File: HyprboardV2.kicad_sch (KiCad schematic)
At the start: 0 parts

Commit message: Crystal Oscilator, Flash Memory done! Started working on the breakout for GPIO pins
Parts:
- added C1, C11, C12, C2, C3, C4, C5, C6, C7, C8, C9: 0.1uF, symbol Device:C
- added C10: 1uF, symbol Device:C
- added C13, C14: 10uF, symbol Device:C
- added C15, C16: 15pF, symbol Device:C
- added J1: USB_C_Receptacle_USB2.0_14P, symbol Connector:USB_C_Receptacle_USB2.0_14P
- added R1, R2: 5.1K, symbol Device:R
- added R3, R4: 27, symbol Device:R
- added R5, R7: 1K, symbol Device:R
- added R6: 10K, symbol Device:R
- added SW1: SW_Push, symbol Switch:SW_Push
- added U1: RP2040, Package_DFN_QFN:QFN-56-1EP_7x7mm_P0.4mm_EP3.2x3.2mm, symbol MCU_RaspberryPi:RP2040
- added U2: NCP1117-3.3_SOT223, Package_TO_SOT_SMD:SOT-223-3_TabPin2, symbol Regulator_Linear:NCP1117-3.3_SOT223
- added U3: W25Q128JVS, Package_SO:SOIC-8_5.3x5.3mm_P1.27mm, symbol Memory_Flash:W25Q128JVS
- added Y1: 12 MHz, symbol Device:Crystal_GND24
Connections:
- new net: J1.A5 (CC1), R1.1
- new net: R3.1, U1.46 (USB_DM)
- new net: R4.1, U1.47 (USB_DP)
- new net: R7.1, SW1.2
- new net: C16.2, R5.1, Y1.1
- new net: C13.2, C14.2
- new net: J1.B5 (CC2), R2.1
- new net +1V1: C10.1, C11.1, C12.1, U1.43 (ADC_AVDD), U1.48 (USB_VDD)
- new net +3V3: C1.1, C14.1, C2.1, C3.1, C4.1, C5.1, C6.1, C7.1, C8.1, C9.1, R6.1, U1.1 (IOVDD), U1.10 (IOVDD), U1.22 (IOVDD), U1.23 (DVDD), U1.33 (IOVDD), U1.42 (IOVDD), U1.44 (VREG_VIN), U1.45 (VREG_VOUT), U1.49 (IOVDD), U1.50 (DVDD), U2.2 (VO), U3.8 (VCC)
- new net GND: C1.2, C10.2, C11.2, C12.2, C15.1, C16.1, C2.2, C3.2, C4.2, C5.2, C6.2, C7.2, C8.2, C9.2, J1.A1 (GND), J1.A12 (GND), J1.B1 (GND), J1.B12 (GND), J1.S1 (SHIELD), R1.2, R2.2, SW1.1, U2.1 (GND), U3.4 (GND), Y1.2 (G), Y1.4 (G)
- new net QSPI_SCLK: U1.52 (QSPI_SCLK), U3.6 (CLK)
- new net QSPI_SD0: U1.53 (QSPI_SD0), U3.5 (DI/IO_{0})
- new net QSPI_SD1: U1.55 (QSPI_SD1), U3.2 (DO/IO_{1})
- new net QSPI_SD2: U1.54 (QSPI_SD2), U3.3 (~{WP}/IO_{2})
- new net QSPI_SD3: U1.51 (QSPI_SD3), U3.7 (~{HOLD}/~{RESET}/IO_{3})
- new net QSPI_SS: R6.2, R7.2, U1.56 (~{QSPI_SS}), U3.1 (~{CS})
- new net USD_D+: J1.A6 (D+), J1.B6 (D+), R3.2
- new net USD_D-: J1.A7 (D-), J1.B7 (D-), R4.2
- new net VBUS: C13.1, J1.A4 (VBUS), J1.A9 (VBUS), J1.B4 (VBUS), J1.B9 (VBUS), U2.3 (VI)
- new net XIN: C15.2, U1.20 (XIN), Y1.3
- new net XOUT: R5.2, U1.21 (XOUT)
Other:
- note added: "CRYSTAL OSCILLATOR"
- note added: "USB"

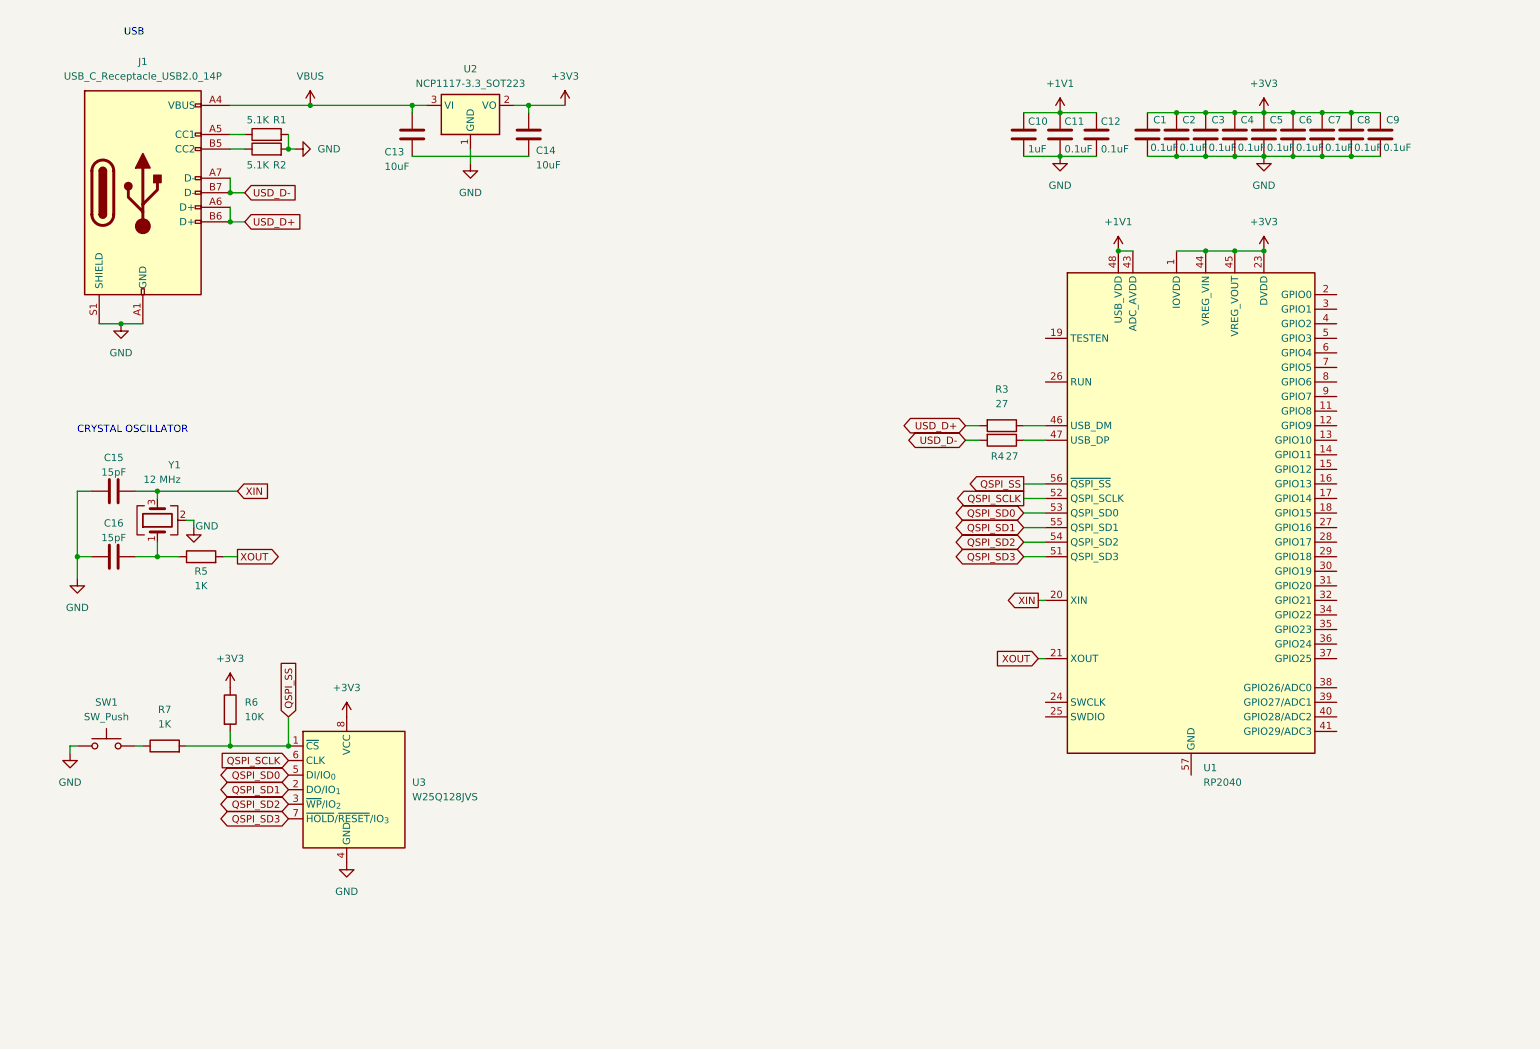
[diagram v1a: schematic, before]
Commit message: Finished up the schematic
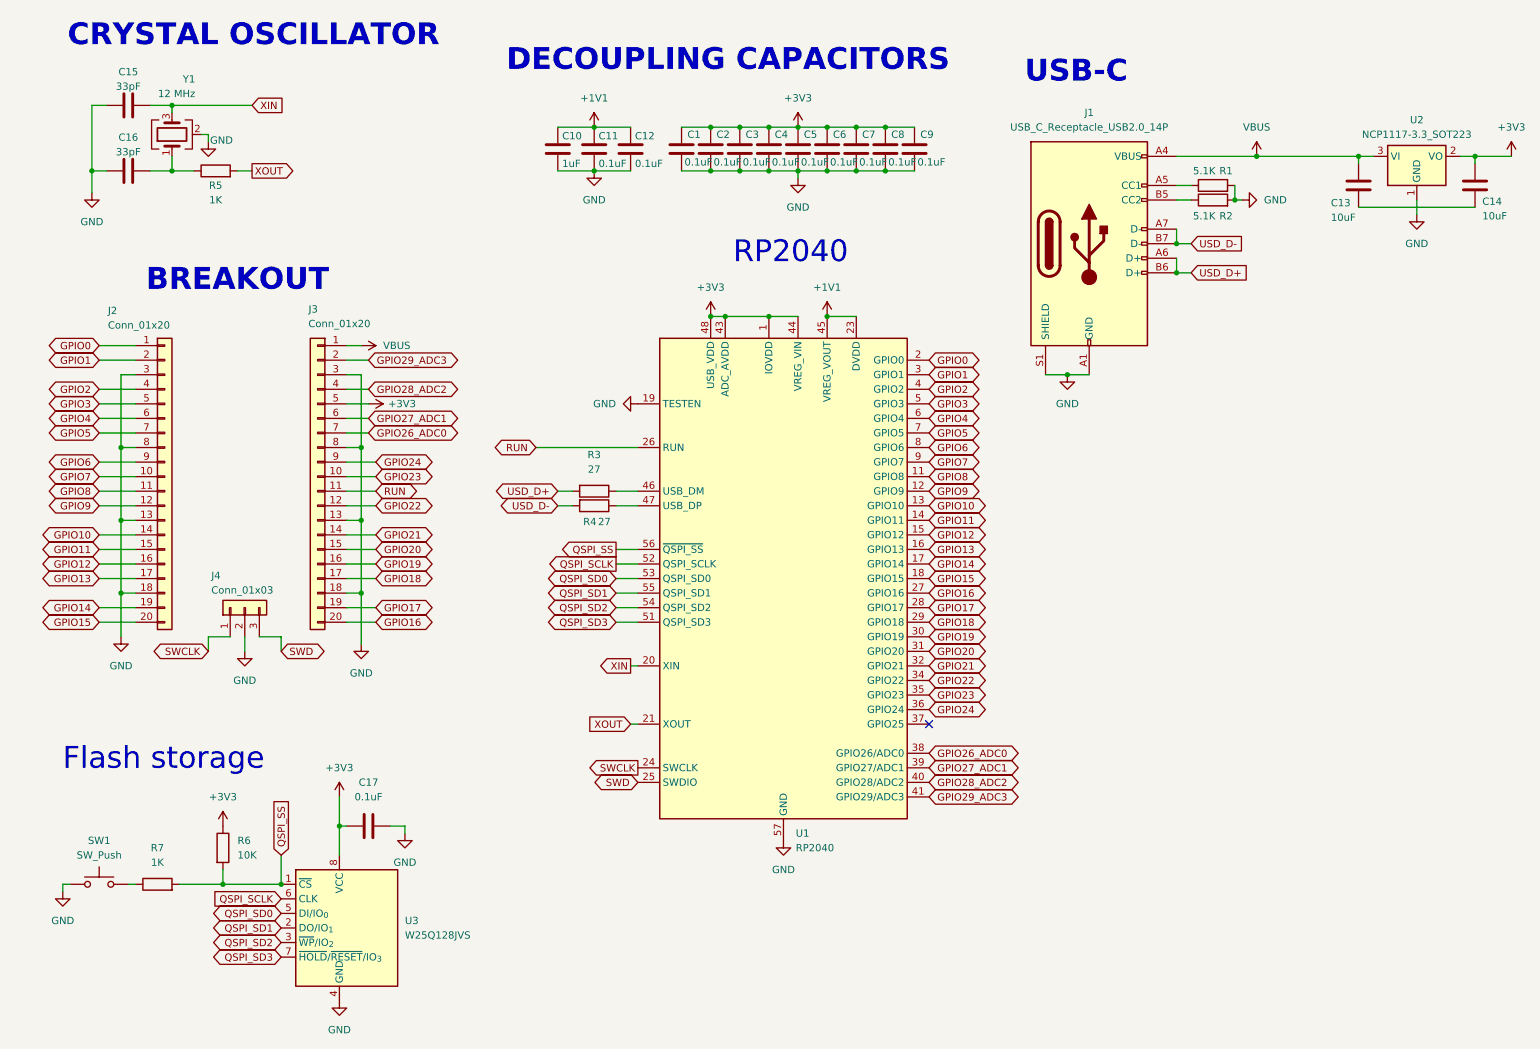
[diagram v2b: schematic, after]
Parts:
- added C17: 0.1uF, Capacitor_SMD:C_0603_1608Metric, symbol Device:C
- added J2, J3: Conn_01x20, Connector_PinHeader_2.54mm:PinHeader_1x20_P2.54mm_Vertical, symbol Connector_Generic:Conn_01x20
- added J4: Conn_01x03, Connector_PinHeader_2.54mm:PinHeader_1x03_P2.54mm_Vertical, symbol Connector_Generic:Conn_01x03
- C1, C10, C11, C12, C2, C3, C4, C5, C6, C7, C8, C9: footprint (none) -> Capacitor_SMD:C_0402_1005Metric
- C13, C14: footprint (none) -> Capacitor_SMD:C_0603_1608Metric
- C15, C16: value 15pF -> 33pF; footprint (none) -> Capacitor_SMD:C_0603_1608Metric
- J1: footprint (none) -> Connector_USB:USB_C_Receptacle_HRO_TYPE-C-31-M-12
- R1, R2, R3, R4, R5, R6, R7: footprint (none) -> Resistor_SMD:R_0402_1005Metric
- SW1: footprint (none) -> Connector_PinHeader_2.54mm:PinHeader_1x20_P2.54mm_Vertical
- Y1: footprint (none) -> Crystal:Crystal_SMD_3225-4Pin_3.2x2.5mm
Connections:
- net +1V1: now also U1.23 (DVDD), U1.45 (VREG_VOUT), U1.50 (DVDD); no longer U1.43 (ADC_AVDD), U1.48 (USB_VDD)
- net +3V3: now also U1.43 (ADC_AVDD), U1.48 (USB_VDD), C17.1, J3.5 (Pin_5); no longer U1.23 (DVDD), U1.45 (VREG_VOUT), U1.50 (DVDD)
- net GND: now also U1.19 (TESTEN), U1.57 (GND), C17.2, J2.13 (Pin_13), J2.18 (Pin_18), J2.3 (Pin_3), J2.8 (Pin_8), J3.13 (Pin_13), J3.18 (Pin_18), J3.3 (Pin_3), J3.8 (Pin_8), J4.2 (Pin_2)
- net VBUS: now also J3.1 (Pin_1)
- net GPIO8: now reaches U1.11 (GPIO8)
- net GPIO8: now also J2.11 (Pin_11)
- net GPIO9: now reaches U1.12 (GPIO9)
- net GPIO9: now also J2.12 (Pin_12)
- net GPIO10: now reaches U1.13 (GPIO10)
- net GPIO10: now also J2.14 (Pin_14)
- net GPIO11: now reaches U1.14 (GPIO11)
- net GPIO11: now also J2.15 (Pin_15)
- net GPIO12: now reaches U1.15 (GPIO12)
- net GPIO12: now also J2.16 (Pin_16)
- net GPIO13: now reaches U1.16 (GPIO13)
- net GPIO13: now also J2.17 (Pin_17)
- net GPIO14: now reaches U1.17 (GPIO14)
- net GPIO14: now also J2.19 (Pin_19)
- net GPIO15: now reaches U1.18 (GPIO15)
- net GPIO15: now also J2.20 (Pin_20)
- net GPIO0: now reaches U1.2 (GPIO0)
- net GPIO0: now also J2.1 (Pin_1)
- net SWCLK: now reaches U1.24 (SWCLK)
- net SWCLK: now also J4.1 (Pin_1)
- net SWD: now reaches U1.25 (SWDIO)
- net SWD: now also J4.3 (Pin_3)
- net RUN: now reaches U1.26 (RUN)
- net RUN: now also J3.11 (Pin_11)
- net GPIO16: now reaches U1.27 (GPIO16)
- net GPIO16: now also J3.20 (Pin_20)
- net GPIO17: now reaches U1.28 (GPIO17)
- net GPIO17: now also J3.19 (Pin_19)
- net GPIO18: now reaches U1.29 (GPIO18)
- net GPIO18: now also J3.17 (Pin_17)
- net GPIO1: now reaches U1.3 (GPIO1)
- net GPIO1: now also J2.2 (Pin_2)
- net GPIO19: now reaches U1.30 (GPIO19)
- net GPIO19: now also J3.16 (Pin_16)
- net GPIO20: now reaches U1.31 (GPIO20)
- net GPIO20: now also J3.15 (Pin_15)
- net GPIO21: now reaches U1.32 (GPIO21)
- net GPIO21: now also J3.14 (Pin_14)
- net GPIO22: now reaches U1.34 (GPIO22)
- net GPIO22: now also J3.12 (Pin_12)
- net GPIO23: now reaches U1.35 (GPIO23)
- net GPIO23: now also J3.10 (Pin_10)
- net GPIO24: now reaches U1.36 (GPIO24)
- net GPIO24: now also J3.9 (Pin_9)
- net GPIO26_ADC0: now reaches U1.38 (GPIO26/ADC0)
- net GPIO26_ADC0: now also J3.7 (Pin_7)
- net GPIO27_ADC1: now reaches U1.39 (GPIO27/ADC1)
- net GPIO27_ADC1: now also J3.6 (Pin_6)
- net GPIO2: now reaches U1.4 (GPIO2)
- net GPIO2: now also J2.4 (Pin_4)
- net GPIO28_ADC2: now reaches U1.40 (GPIO28/ADC2)
- net GPIO28_ADC2: now also J3.4 (Pin_4)
- net GPIO29_ADC3: now reaches U1.41 (GPIO29/ADC3)
- net GPIO29_ADC3: now also J3.2 (Pin_2)
- net GPIO3: now reaches U1.5 (GPIO3)
- net GPIO3: now also J2.5 (Pin_5)
- net GPIO4: now reaches U1.6 (GPIO4)
- net GPIO4: now also J2.6 (Pin_6)
- net GPIO5: now reaches U1.7 (GPIO5)
- net GPIO5: now also J2.7 (Pin_7)
- net GPIO6: now reaches U1.8 (GPIO6)
- net GPIO6: now also J2.9 (Pin_9)
- net GPIO7: now reaches U1.9 (GPIO7)
- net GPIO7: now also J2.10 (Pin_10)
- no-connect marks 0 -> 1
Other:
- note added: "BREAKOUT"
- note added: "DECOUPLING CAPACITORS"
- note added: "Flash storage"
- note added: "RP2040"
- note added: "USB-C"
- note removed: "USB"
- moved on the sheet: C1, C10, C11, C12, C13, C14, C15, C16, C2, C3, C4, C5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
